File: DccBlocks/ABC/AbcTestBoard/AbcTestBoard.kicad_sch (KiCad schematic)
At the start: 25 parts, among them J1 Conn_02x02_Odd_Even, J3 Conn_01x02, J5 Conn_01x02, J6 Conn_01x02, Q1 PSMN022, Q2 PSMN022, Q3 PSMN022, Q4 PSMN022, U1 VO615A, U2 VO615A

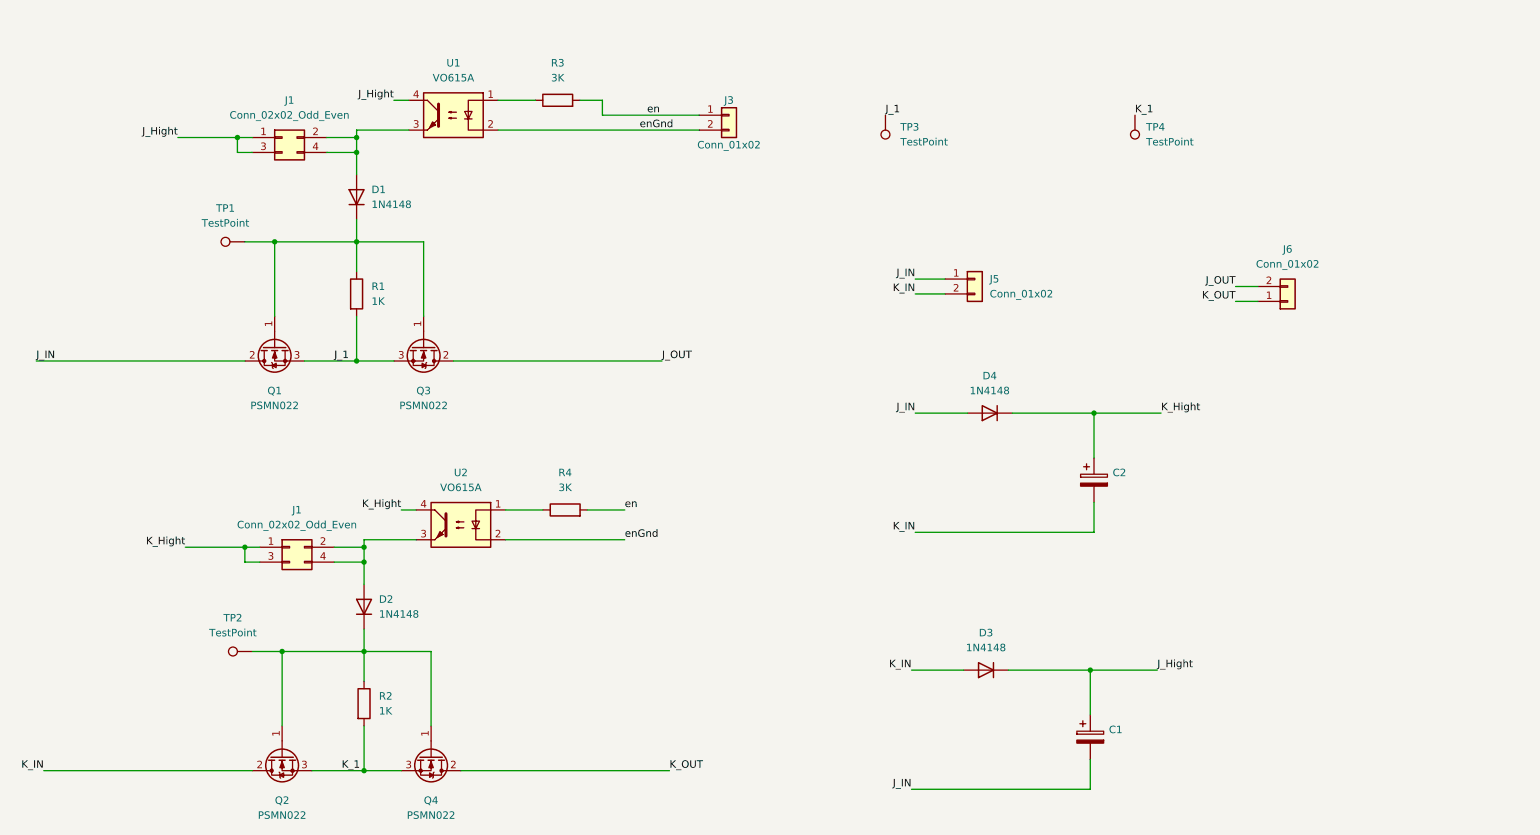
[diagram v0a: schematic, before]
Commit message: Version PMos switch
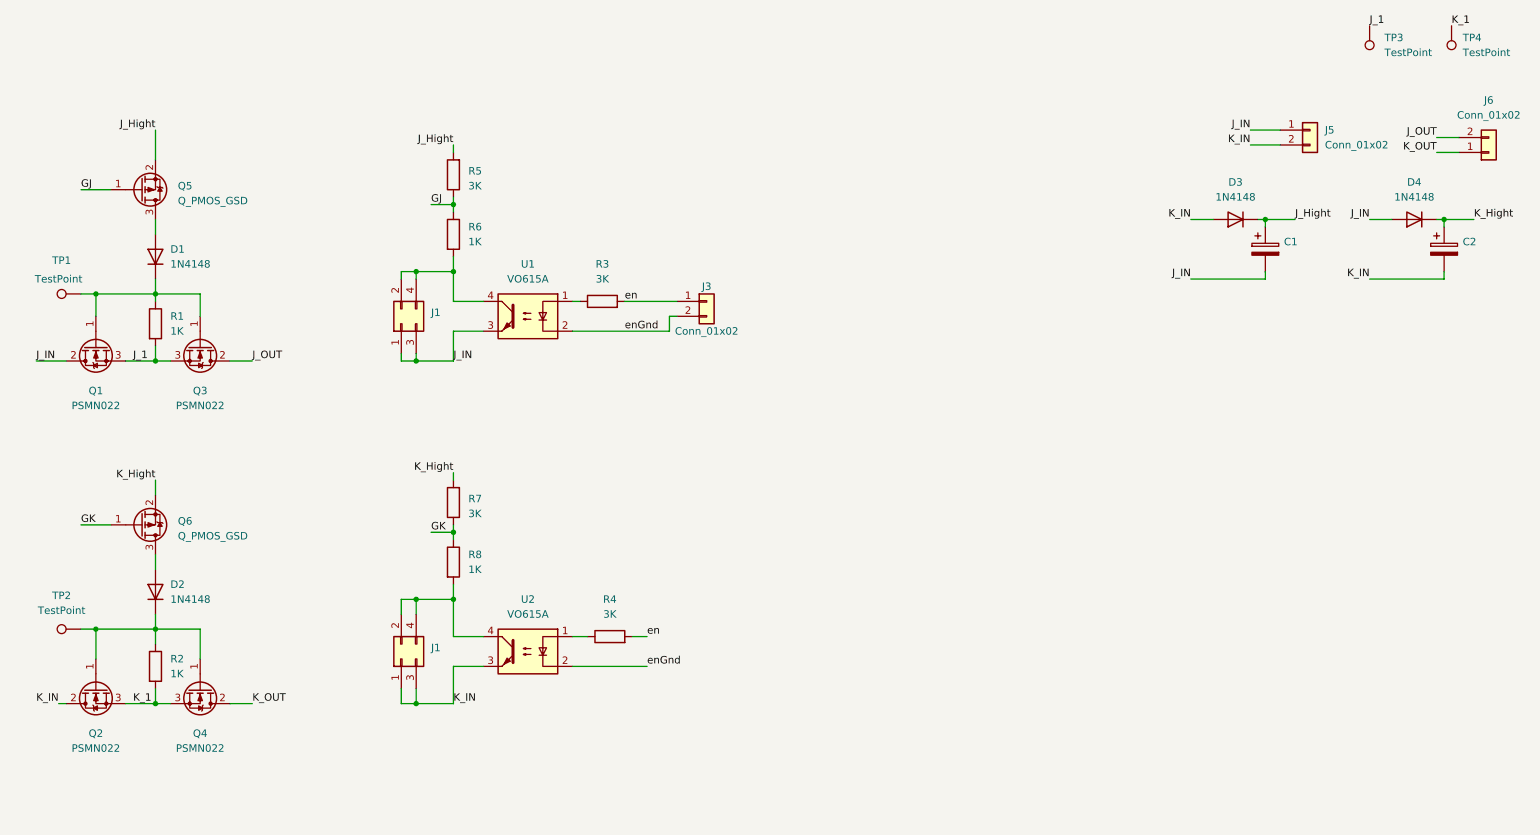
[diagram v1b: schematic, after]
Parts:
- added Q5, Q6: Q_PMOS_GSD, Package_TO_SOT_SMD:SOT-23, symbol Device:Q_PMOS_GSD
- added R5, R7: 3K, Resistor_SMD:R_1206_3216Metric_Pad1.30x1.75mm_HandSolder, symbol Device:R
- added R6, R8: 1K, Resistor_SMD:R_1206_3216Metric_Pad1.30x1.75mm_HandSolder, symbol Device:R
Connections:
- net J_Hight: now also Q5.2 (S), R5.2; no longer J1.1 (Pin_1), J1.3 (Pin_3), U1.4
- net J_IN: now also J1.1 (Pin_1), J1.3 (Pin_3), U1.3
- net K_Hight: now also Q6.2 (S), R7.2; no longer J1.1 (Pin_1), J1.3 (Pin_3), U2.4
- net K_IN: now also J1.1 (Pin_1), J1.3 (Pin_3), U2.3
- net at J1.2 (Pin_2), J1.4 (Pin_4): now also U1.4, R6.2; no longer D1.2 (A), U1.3
- net at J1.2 (Pin_2), J1.4 (Pin_4): now also U2.4, R8.2; no longer D2.2 (A), U2.3
- new net: D2.2 (A), Q6.3 (D)
- new net: D1.2 (A), Q5.3 (D)
- new net GJ: Q5.1 (G), R5.1, R6.1
- new net GK: Q6.1 (G), R7.1, R8.1
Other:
- moved on the sheet: C1, C2, D1, D2, D3, D4, J1, J3, J5, J6, Q1, Q2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
